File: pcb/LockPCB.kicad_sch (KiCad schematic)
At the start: 0 parts

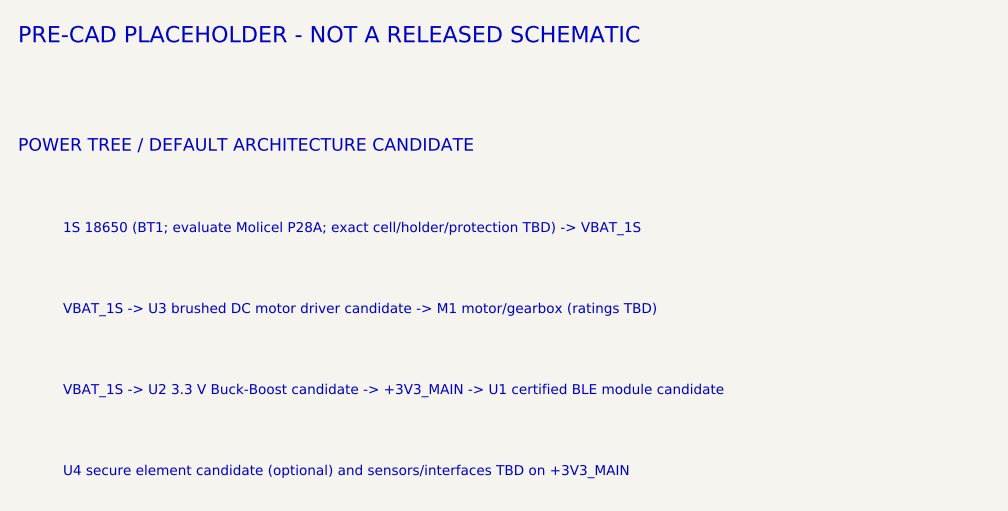
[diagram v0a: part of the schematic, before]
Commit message: Reset CAD handoff to confirmed mechanical baseline
Co-authored-by: arena-agent <297053741+arena-agent@users.noreply.github.com>
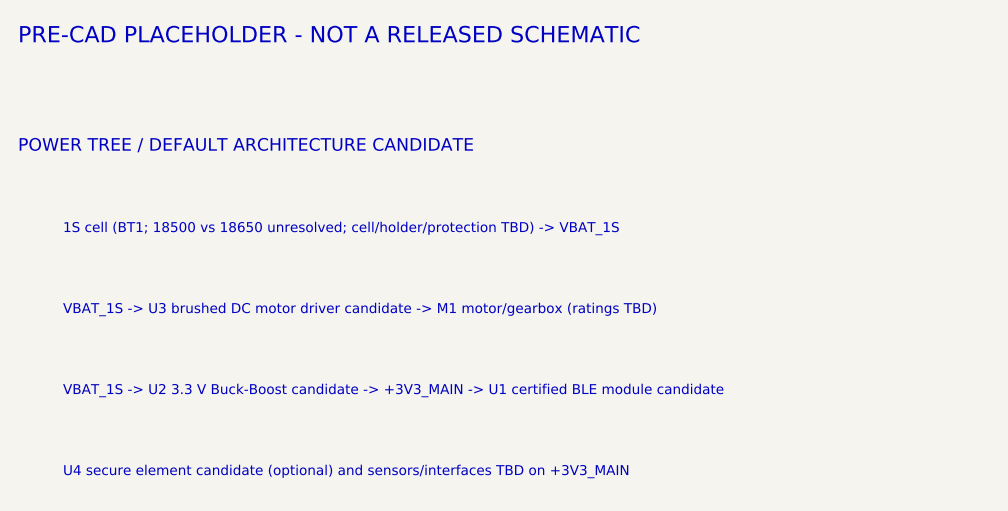
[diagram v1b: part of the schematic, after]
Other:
- note added: "1S cell (BT1; 18500 vs 18650 unresolved; cell/holder/protection TBD) -> VBAT_1S"
- note removed: "1S 18650 (BT1; evaluate Molicel P28A; exact cell/holder/protection TBD) -> VBAT_1S"
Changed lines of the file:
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@@
   (text "PRE-CAD PLACEHOLDER - NOT A RELEASED SCHEMATIC" (at 25 28 0) (effects (font (size 1.8 1.8)) (justify left bottom)))
   (text "POWER TREE / DEFAULT ARCHITECTURE CANDIDATE" (at 25 40 0) (effects (font (size 1.4 1.4)) (justify left bottom)))
-  (text "1S 18650 (BT1; evaluate Molicel P28A; exact cell/holder/protection TBD) -> VBAT_1S" (at 30 49 0) (effects (font (size 1.1 1.1)) (justify left bottom)))
+  (text "1S cell (BT1; 18500 vs 18650 unresolved; cell/holder/protection TBD) -> VBAT_1S" (at 30 49 0) (effects (font (size 1.1 1.1)) (justify left bottom)))
   (text "VBAT_1S -> U3 brushed DC motor driver candidate -> M1 motor/gearbox (ratings TBD)" (at 30 58 0) (effects (font (size 1.1 1.1)) (justify left bottom)))
   (text "VBAT_1S -> U2 3.3 V Buck-Boost candidate -> +3V3_MAIN -> U1 certified BLE module candidate" (at 30 67 0) (effects (font (size 1.1 1.1)) (justify left bottom)))
